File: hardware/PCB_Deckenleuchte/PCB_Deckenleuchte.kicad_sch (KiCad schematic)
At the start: 1 part, among them U1 IRM-20-3.3

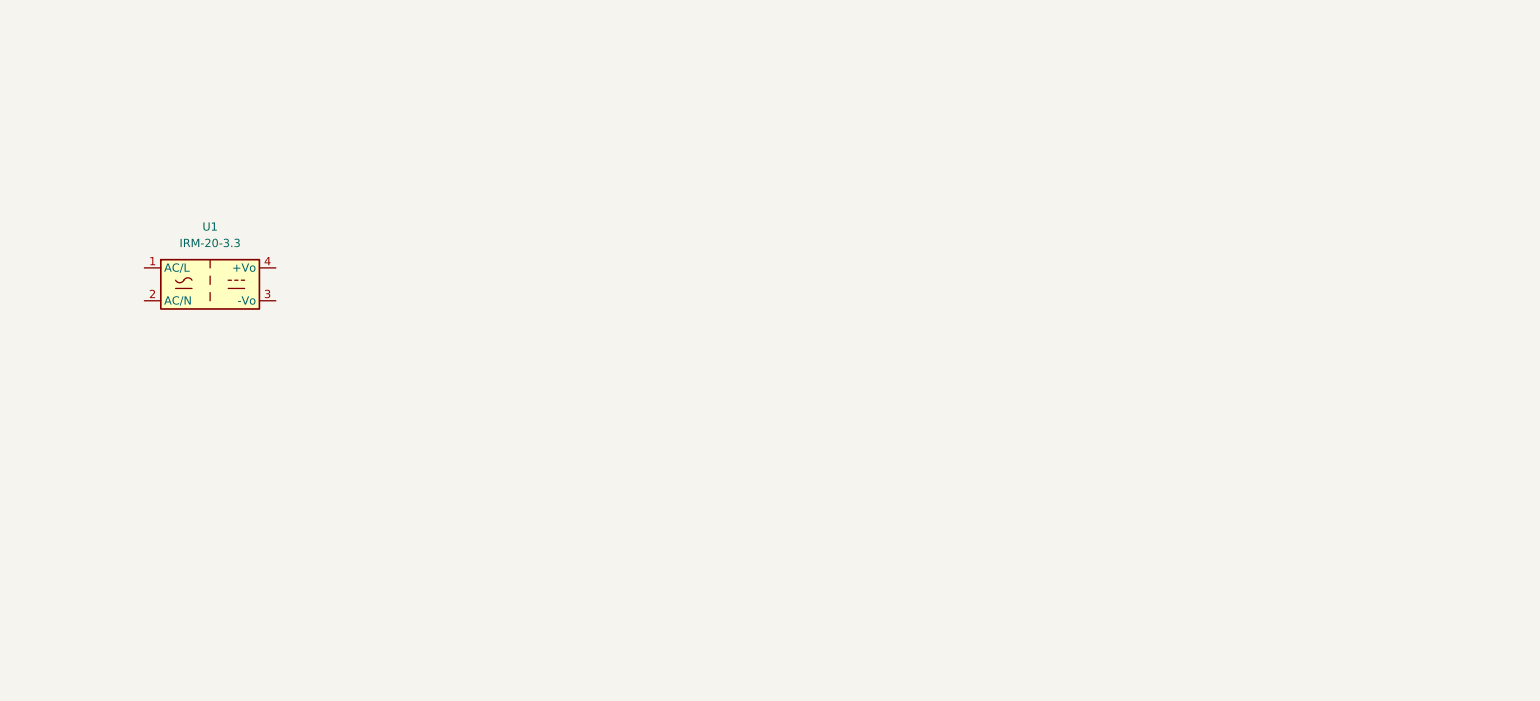
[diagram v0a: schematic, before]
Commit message: Add files via upload
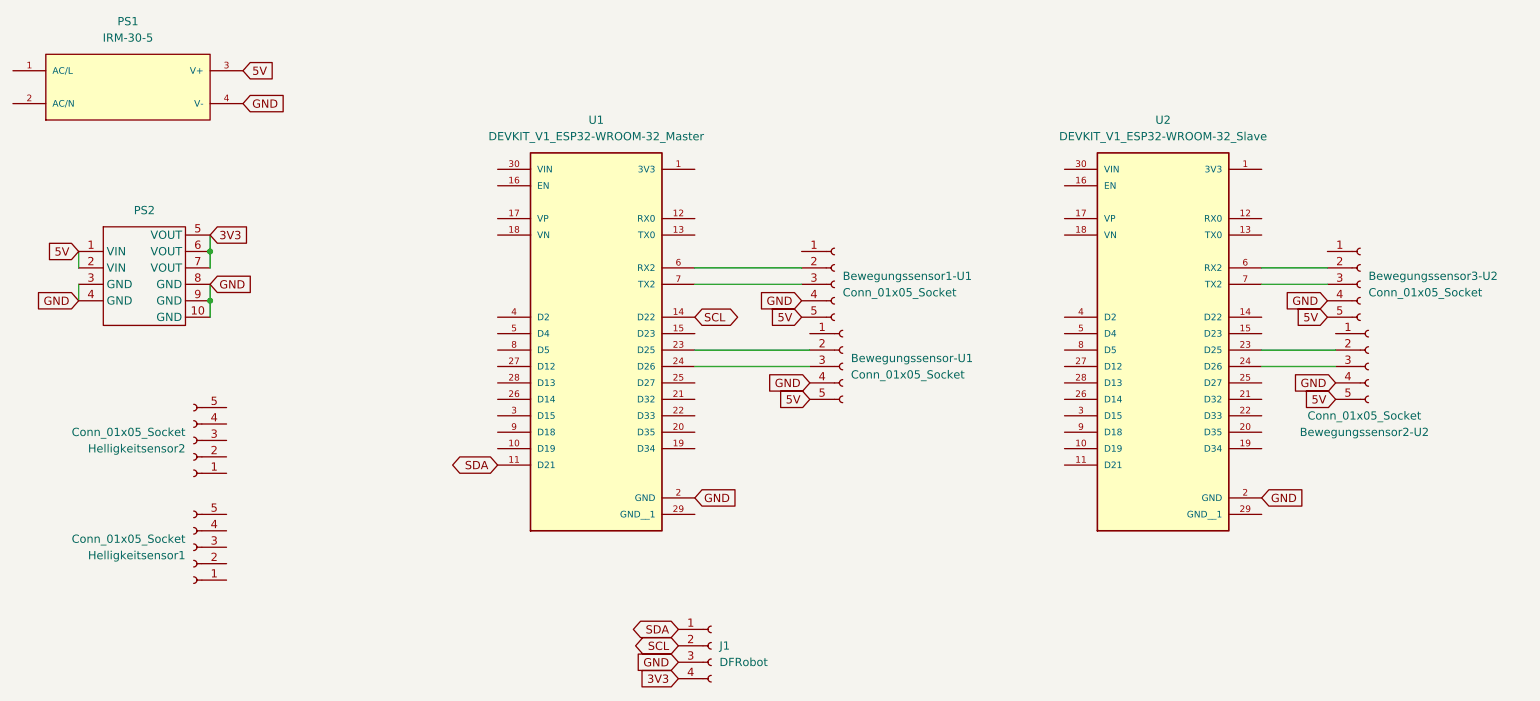
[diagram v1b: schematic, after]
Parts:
- removed U1: IRM-20-3.3, Converter_ACDC:Converter_ACDC_MeanWell_IRM-20-xx_THT, symbol Converter_ACDC:IRM-20-3.3
- added Bewegungssensor-U1, Bewegungssensor1-U1, Bewegungssensor2-U2, Bewegungssensor3-U2, Helligkeitsensor1, Helligkeitsensor2: Conn_01x05_Socket, Connector_JST:JST_XH_B5B-XH-A_1x05_P2.50mm_Vertical, symbol Connector:Conn_01x05_Socket
- added J1: DFRobot, Connector_JST:JST_PH_B4B-PH-K_1x04_P2.00mm_Vertical, symbol Connector:Conn_01x04_Socket
- added PS1: IRM-30-5, IRM-30-5:CONV_IRM-30-5, symbol IRM-30-5:IRM-30-5
- added PS2: (no value), third_party_components:DC5-36-TO-DC3V3-5, symbol third_party_components:DC5-36-TO-DC3V3-5
- added U1: DEVKIT_V1_ESP32-WROOM-32_Master, DEVKIT_V1_ESP32-WROOM-32:MODULE_DEVKIT_V1_ESP32-WROOM-32, symbol DEVKIT_V1_ESP32-WROOM-32:DEVKIT_V1_ESP32-WROOM-32
- added U2: DEVKIT_V1_ESP32-WROOM-32_Slave, DEVKIT_V1_ESP32-WROOM-32:MODULE_DEVKIT_V1_ESP32-WROOM-32, symbol DEVKIT_V1_ESP32-WROOM-32:DEVKIT_V1_ESP32-WROOM-32
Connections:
- new net: Bewegungssensor3-U2.2 (Pin_2), U2.6 (RX2)
- new net: Bewegungssensor3-U2.3 (Pin_3), U2.7 (TX2)
- new net: Bewegungssensor2-U2.2 (Pin_2), U2.23 (D25)
- new net: Bewegungssensor2-U2.3 (Pin_3), U2.24 (D26)
- new net: Bewegungssensor-U1.2 (Pin_2), U1.23 (D25)
- new net: Bewegungssensor-U1.3 (Pin_3), U1.24 (D26)
- new net: Bewegungssensor1-U1.2 (Pin_2), U1.6 (RX2)
- new net: Bewegungssensor1-U1.3 (Pin_3), U1.7 (TX2)
- new net 3V3: J1.4 (Pin_4), PS2.5 (VOUT), PS2.6 (VOUT), PS2.7 (VOUT)
- new net 5V: Bewegungssensor-U1.5 (Pin_5), Bewegungssensor1-U1.5 (Pin_5), Bewegungssensor2-U2.5 (Pin_5), Bewegungssensor3-U2.5 (Pin_5), PS1.3 (V+), PS2.1 (VIN), PS2.2 (VIN)
- new net GND: Bewegungssensor-U1.4 (Pin_4), Bewegungssensor1-U1.4 (Pin_4), Bewegungssensor2-U2.4 (Pin_4), Bewegungssensor3-U2.4 (Pin_4), J1.3 (Pin_3), PS1.4 (V-), PS2.10 (GND), PS2.3 (GND), PS2.4 (GND), PS2.8 (GND), PS2.9 (GND), U1.2 (GND), U2.2 (GND)
- new net SCL: J1.2 (Pin_2), U1.14 (D22)
- new net SDA: J1.1 (Pin_1), U1.11 (D21)
